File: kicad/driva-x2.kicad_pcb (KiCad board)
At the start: 4 copper layers, 100 x 50 mm, 199 parts, among them J1 CONN_HALL_1, J10 CONN_SPI_2, J11 CONN_CAN, J12 CONN_POWER, J2 CONN_PROG, J3 CONN_USB_OTG, J4 CONN_I2C, J5 CONN_POWER2, J6 CONN_SERVO, J8 CONN_SPI_1, J9 CONN_HALL_2, Q1 TPH1R403NL, Q10 TPH1R403NL, Q11 TPH1R403NL, Q12 TPH1R403NL, Q2 TPH1R403NL, Q3 TPH1R403NL, Q4 TPH1R403NL, Q5 TPH1R403NL, Q6 TPH1R403NL, Q7 TPH1R403NL, Q8 TPH1R403NL, Q9 TPH1R403NL, SW1 push, SW2 push, SW3 push, U1 INA240A2PW, U10 L6387ED, U11 INA240A2PW, U12 L6387ED, U13 AMS1117-3.3, U14 TJA1051T-3, U15 STM32F405RGTx, U2 L6387ED, U3 INA240A2PW, U4 L6387ED, U5 INA240A2PW, U6 L6387ED, U7 INA240A2PW, U8 L6387ED, U9 INA240A2PW

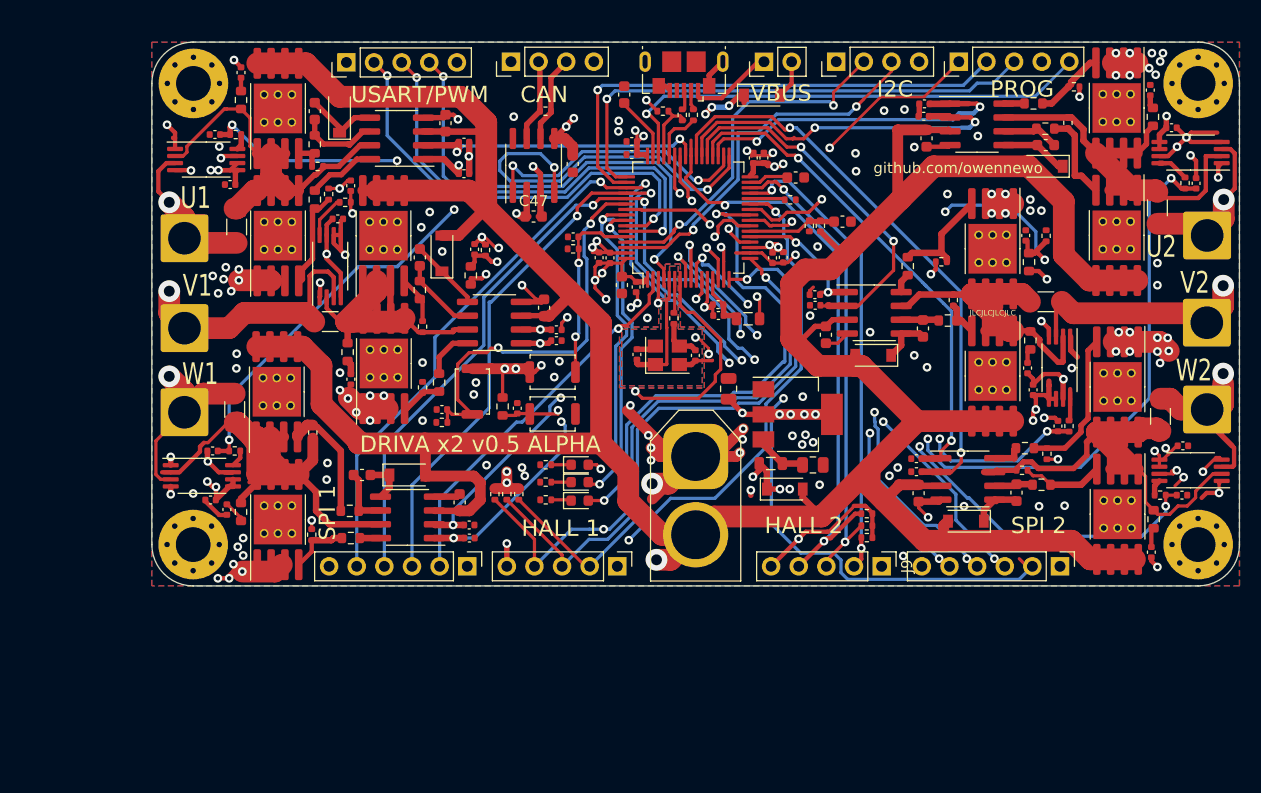
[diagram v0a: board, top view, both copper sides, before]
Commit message: Adding 0.9 version
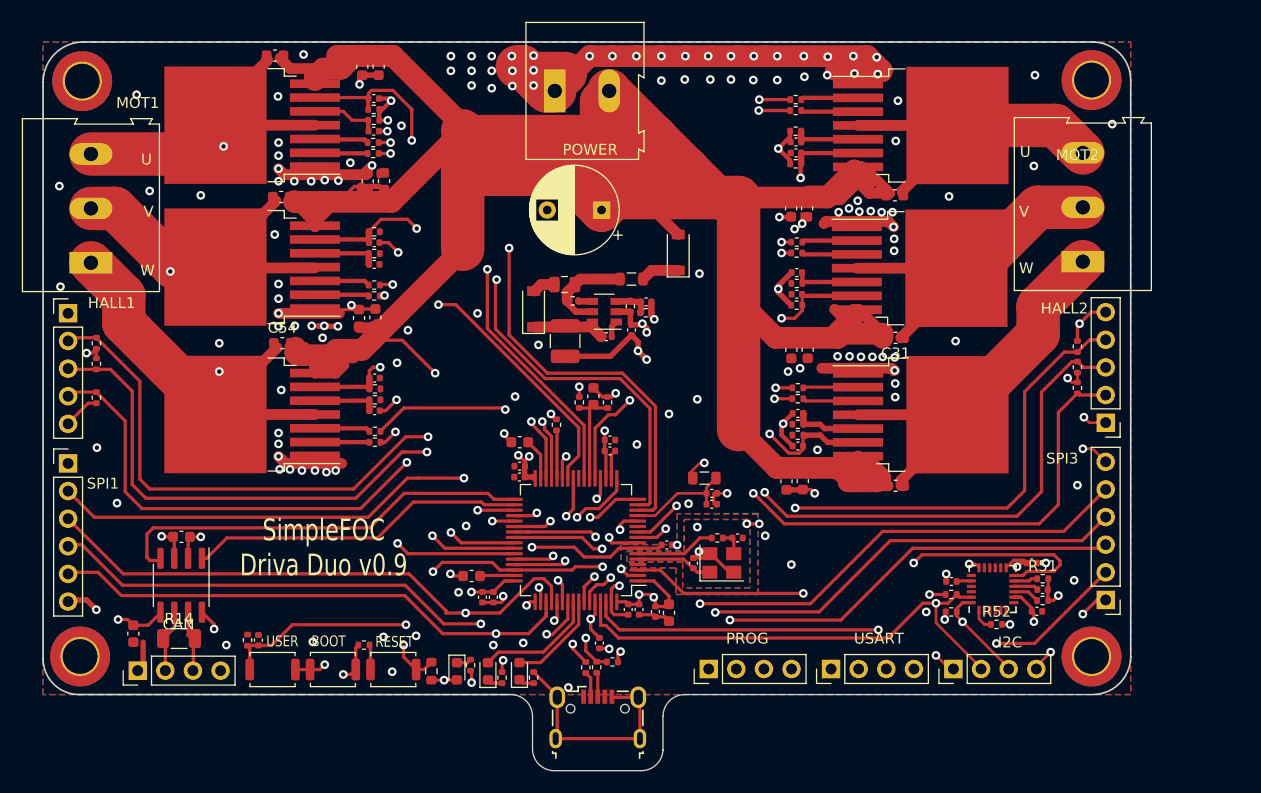
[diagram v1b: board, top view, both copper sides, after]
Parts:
- removed C62, C64, C66, C68: 100n, Capacitor_SMD:C_0402_1005Metric
- removed C63, C65, C67: 1n, Capacitor_SMD:C_0402_1005Metric
- removed D10: BLUE, LED_SMD:LED_0603_1608Metric
- removed D11, D6, D7: b5819w, Diode_SMD:D_SOD-123
- removed D8: RED, LED_SMD:LED_0603_1608Metric
- removed D9: GREEN, LED_SMD:LED_0603_1608Metric
- removed H10: PAD_W_2, Connector_Wire:SolderWire-2.5sqmm_1x01_D2.4mm_OD4.4mm
- removed H5: PAD_U_1, Connector_Wire:SolderWire-2.5sqmm_1x01_D2.4mm_OD4.4mm
- removed H6: PAD_V_1, Connector_Wire:SolderWire-2.5sqmm_1x01_D2.4mm_OD4.4mm
- removed H7: PAD_W_1, Connector_Wire:SolderWire-2.5sqmm_1x01_D2.4mm_OD4.4mm
- removed H8: PAD_U_2, Connector_Wire:SolderWire-2.5sqmm_1x01_D2.4mm_OD4.4mm
- removed H9: PAD_V_2, Connector_Wire:SolderWire-2.5sqmm_1x01_D2.4mm_OD4.4mm
- removed Q1, Q10, Q11, Q12, Q2, Q3, Q4, Q5, Q6, Q7, Q8, Q9: TPH1R403NL, Package_SO:SOP-8-1EP_4.57x4.57mm_P1.27mm_EP4.57x4.45mm_ThermalVias
- removed R53: 3K3, Resistor_SMD:R_0402_1005Metric
- removed R54: 4k7, Resistor_SMD:R_0402_1005Metric
- removed R55: 10k, Resistor_SMD:R_0402_1005Metric
- removed R56, R57, R58, R59, R60, R61, R62, R63, R64: 1K, Resistor_SMD:R_0402_1005Metric
- removed TH1, TH2: Thermistor, Resistor_SMD:R_0603_1608Metric
- removed U11: INA240A2PW, Package_SO:TSSOP-8_4.4x3mm_P0.65mm
- removed U12: L6387ED, Package_SO:SOIC-8_3.9x4.9mm_P1.27mm
- removed U13: AMS1117-3.3, Package_TO_SOT_SMD:SOT-223-3_TabPin2
- removed U14: TJA1051T-3, Package_SO:SOIC-8_3.9x4.9mm_P1.27mm
- removed U15: STM32F405RGTx, Package_QFP:LQFP-64_10x10mm_P0.5mm
- added J7: CONN_SPI_1, Connector_PinHeader_2.54mm:PinHeader_1x06_P2.54mm_Vertical, F.Cu at (64.3, 68.8)
- added L1: 2.2uh, Inductor_SMD:L_1210_3225Metric, F.Cu at (110.0, 57.5)
- C1: value 1u -> 10u
- C10, C20, C25, C30, C5, C53: value 10n -> 100n
- C11, C6: value 1u -> 100n; footprint Capacitor_SMD:C_0603_1608Metric -> Capacitor_SMD:C_0402_1005Metric
- C12: value 100p -> 10u
- C13: value 100p -> 4.7u+; footprint Capacitor_SMD:C_0402_1005Metric -> Capacitor_SMD:C_0805_2012Metric
- C14, C4, C9: value 470n -> 100n; footprint Capacitor_SMD:C_0603_1608Metric -> Capacitor_SMD:C_0402_1005Metric
- C16: value 1u -> 12p; footprint Capacitor_SMD:C_0603_1608Metric -> Capacitor_SMD:C_0402_1005Metric
- C17: value 100p -> 12p
- C18, C2, C3, C7, C8: value 100p -> 100n
- C19: value 470n -> 2.2u
- C21: value 1u -> 2.2u
- C22, C23: value 100p -> 2.2u; footprint Capacitor_SMD:C_0402_1005Metric -> Capacitor_SMD:C_0603_1608Metric
- C24: value 470n -> 10u
- C26: value 1u -> 220n+
- C27: value 100p -> 100n+; footprint Capacitor_SMD:C_0402_1005Metric -> Capacitor_SMD:C_0603_1608Metric
- C28: value 100p -> 220n+; footprint Capacitor_SMD:C_0402_1005Metric -> Capacitor_SMD:C_0603_1608Metric
- C29: value 470n -> 1n; footprint Capacitor_SMD:C_0603_1608Metric -> Capacitor_SMD:C_0402_1005Metric
- C31, C54: value 10u -> 220n+
- C32, C37: value 100n -> 100n+; footprint Capacitor_SMD:C_0402_1005Metric -> Capacitor_SMD:C_0603_1608Metric
- C33, C36, C38, C49, C56: value 100n -> 220n+; footprint Capacitor_SMD:C_0402_1005Metric -> Capacitor_SMD:C_0603_1608Metric
- C34, C39: value 100n -> 1n
- C41, C42: value 10u -> 100n; footprint Capacitor_SMD:C_0805_2012Metric -> Capacitor_SMD:C_0402_1005Metric
- C43: value 100n -> 2.2n
- C44: value 10n -> 220n+; footprint Capacitor_SMD:C_0402_1005Metric -> Capacitor_SMD:C_0603_1608Metric
- C45: value 12p -> 100n+; footprint Capacitor_SMD:C_0402_1005Metric -> Capacitor_SMD:C_0603_1608Metric
- C46: value 12p -> 220n+; footprint Capacitor_SMD:C_0402_1005Metric -> Capacitor_SMD:C_0603_1608Metric
- C47, C52: value 2.2u -> 1n; footprint Capacitor_SMD:C_0603_1608Metric -> Capacitor_SMD:C_0402_1005Metric
- C50: value 2.2u -> 100n+
- C51: value 2.2u -> 220n+
- C55: value 10n -> 100n+; footprint Capacitor_SMD:C_0402_1005Metric -> Capacitor_SMD:C_0603_1608Metric
- C59: value 1n -> 33p
- C60: value 100n -> 1000u+; footprint Capacitor_SMD:C_0402_1005Metric -> Capacitor_THT:CP_Radial_D8.0mm_P5.00mm
- C61: value 1n -> 10n
- D2: value b5819w -> RED; footprint Diode_SMD:D_SOD-123 -> LED_SMD:LED_0603_1608Metric
- D3: value b5819w -> GREEN; footprint Diode_SMD:D_SOD-123 -> LED_SMD:LED_0603_1608Metric
- D4: value b5819w -> BLUE; footprint Diode_SMD:D_SOD-123 -> LED_SMD:LED_0603_1608Metric
- H1, H2, H3, H4: footprint MountingHole:MountingHole_3.2mm_M3_Pad_Via -> MountingHole:MountingHole_3.2mm_M3_ISO14580_Pad_TopBottom
- J10: value CONN_SPI_2 -> CONN_CAN; footprint Connector_PinHeader_2.54mm:PinHeader_1x06_P2.54mm_Vertical -> Connector_PinHeader_2.54mm:PinHeader_1x04_P2.54mm_Vertical
- J11: value CONN_CAN -> CONN_PWR; footprint Connector_PinHeader_2.54mm:PinHeader_1x04_P2.54mm_Vertical -> TerminalBlock:TerminalBlock_Altech_AK300-2_P5.00mm
- J12: value CONN_POWER -> CONN_SERIAL; footprint Connector_AMASS:AMASS_XT60-M_1x02_P7.20mm_Vertical -> Connector_PinHeader_2.54mm:PinHeader_1x04_P2.54mm_Vertical
- J2: footprint Connector_PinHeader_2.54mm:PinHeader_1x05_P2.54mm_Vertical -> Connector_PinHeader_2.54mm:PinHeader_1x04_P2.54mm_Vertical
- J3: footprint Connector_USB:USB_Micro-B_GCT_USB3076-30-A -> Connector_USB:USB_Micro-B_Wuerth_629105150521
- J4: value CONN_I2C -> CONN_MOT_1; footprint Connector_PinHeader_2.54mm:PinHeader_1x04_P2.54mm_Vertical -> TerminalBlock:TerminalBlock_Altech_AK300-3_P5.00mm
- J5: value CONN_POWER2 -> CONN_SERIAL; footprint Connector_PinHeader_2.54mm:PinHeader_1x02_P2.54mm_Vertical -> Connector_PinHeader_2.54mm:PinHeader_1x04_P2.54mm_Vertical
- J6: value CONN_SERVO -> CONN_MOT_2; footprint Connector_PinHeader_2.54mm:PinHeader_1x05_P2.54mm_Vertical -> TerminalBlock:TerminalBlock_Altech_AK300-3_P5.00mm
- J8: value CONN_SPI_1 -> CONN_SPI_2
- R10: value 33 -> 220; footprint Resistor_SMD:R_0603_1608Metric -> Resistor_SMD:R_0402_1005Metric
- R11: value 10k -> 2K2; footprint Resistor_SMD:R_0402_1005Metric -> Resistor_SMD:R_0603_1608Metric
- R12, R30, R42: value 0.002R @1W -> 10k; footprint Resistor_SMD:R_1206_3216Metric -> Resistor_SMD:R_0402_1005Metric
- R13, R22, R25, R34, R37: value 33 -> 10k; footprint Resistor_SMD:R_0603_1608Metric -> Resistor_SMD:R_0402_1005Metric
- R14: value 1 -> 120R+; footprint Resistor_SMD:R_0603_1608Metric -> Resistor_SMD:R_1206_3216Metric
- R15: value 10k -> 33K
- R16: value 33 -> 3K3; footprint Resistor_SMD:R_0603_1608Metric -> Resistor_SMD:R_0402_1005Metric
- R18: value 0.002R @1W -> 1K; footprint Resistor_SMD:R_1206_3216Metric -> Resistor_SMD:R_0402_1005Metric
- R19: value 33 -> 1K; footprint Resistor_SMD:R_0603_1608Metric -> Resistor_SMD:R_0402_1005Metric
- R20: value 1 -> 1K; footprint Resistor_SMD:R_0603_1608Metric -> Resistor_SMD:R_0402_1005Metric
- R23, R27, R35, R39: value 10k -> 1k
- R24, R36: value 0.002R @1W -> 510R; footprint Resistor_SMD:R_1206_3216Metric -> Resistor_SMD:R_0402_1005Metric
- R26, R38: value 1 -> 10k; footprint Resistor_SMD:R_0603_1608Metric -> Resistor_SMD:R_0402_1005Metric
- R28, R40: value 33 -> 510R; footprint Resistor_SMD:R_0603_1608Metric -> Resistor_SMD:R_0402_1005Metric
- R31, R43: value 33 -> 1k; footprint Resistor_SMD:R_0603_1608Metric -> Resistor_SMD:R_0402_1005Metric
- R32, R44: value 1 -> 510R; footprint Resistor_SMD:R_0603_1608Metric -> Resistor_SMD:R_0402_1005Metric
- R45: value 10k -> 400K
- R46: value 220 -> 4.7k
- R47: value 2K2 -> 4.7k; footprint Resistor_SMD:R_0603_1608Metric -> Resistor_SMD:R_0402_1005Metric
- R48: value 10k -> 4.7k
- R49: value 10k -> 120k
- R50: value 220 -> 39k
- R51: value 33K -> 10k
- R52: value 4k7 -> 10k
- U1: value INA240A2PW -> mp2451dt; footprint Package_SO:TSSOP-8_4.4x3mm_P0.65mm -> Package_TO_SOT_SMD:SOT-23-6
- U10, U4, U6, U8: value L6387ED -> IFX007T; footprint Package_SO:SOIC-8_3.9x4.9mm_P1.27mm -> Package_TO_SOT_SMD:TO-263-7_TabPin8
- U2: value L6387ED -> TJA1051T-3
- U3: value INA240A2PW -> STM32F405RGTx; footprint Package_SO:TSSOP-8_4.4x3mm_P0.65mm -> Package_QFP:LQFP-64_10x10mm_P0.5mm
- U5, U9: value INA240A2PW -> IFX007T; footprint Package_SO:TSSOP-8_4.4x3mm_P0.65mm -> Package_TO_SOT_SMD:TO-263-7_TabPin8
- U7: value INA240A2PW -> MPU-6050; footprint Package_SO:TSSOP-8_4.4x3mm_P0.65mm -> Sensor_Motion:InvenSense_QFN-24_4x4mm_P0.5mm
- moved H1 102.6 mm to (65.6, 33.6)
- moved R14 101.6 mm to (74.5, 84.8), turned to 0 degrees
- moved H3 98.0 mm to (158.4, 86.5)
- moved J10 85.3 mm to (70.7, 87.8), turned to 90 degrees
- moved U2 84.6 mm to (74.7, 80.0), turned to 270 degrees
- moved U7 82.4 mm to (149.3, 80.3), turned to 90 degrees
- moved R13 79.2 mm to (91.5, 85.5)
- moved C58 77.8 mm to (92.5, 63.9)
- moved C57 77.6 mm to (92.5, 60.9), turned to 0 degrees
- moved R11 77.2 mm to (97.7, 87.8)
- moved C5 77.1 mm to (102.4, 81.0)
- moved R17 72.0 mm to (80.8, 85.0), turned to 90 degrees
- moved J4 71.0 mm to (66.4, 50.3)
- moved J6 70.1 mm to (157.6, 50.2)
- moved R18 62.6 mm to (101.3, 87.3), turned to 90 degrees
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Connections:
- C1 pad 1: Net-(C1-Pad1) -> GND
- C1 pad 2: Net-(C1-Pad2) -> +3V3
- C10 pad 1: Net-(C10-Pad1) -> GND
- C10 pad 2: GND -> +3V3
- C12 pad 1: /driver_2/HIN_W -> GND
- C12 pad 2: GND -> +3V3
- C13 pad 1: /driver_2/LIN_W -> GND
- C13 pad 2: GND -> Net-(C13-Pad2)
- C14 pad 1: VCC -> GND
- C14 pad 2: GND -> +3.3VA
- C15 pad 1: Net-(C15-Pad1) -> GND
- C15 pad 2: GND -> +3.3VA
- C16 pad 1: Net-(C16-Pad1) -> HSE_IN
- C16 pad 2: Net-(C16-Pad2) -> GND
- C17 pad 1: /driver_1/HIN_U -> Net-(C17-Pad1)
- C18 pad 1: /driver_1/LIN_U -> BOOT0
- C19 pad 1: VCC -> GND
- C19 pad 2: GND -> +3V3
- C2 pad 1: /driver_2/HIN_U -> GND
- C2 pad 2: GND -> +3V3
- C20 pad 1: Net-(C20-Pad1) -> NRST
- C21 pad 1: Net-(C21-Pad1) -> GND
- C21 pad 2: Net-(C21-Pad2) -> +3V3
- C22 pad 1: /driver_1/HIN_V -> Net-(C22-Pad1)
- C23 pad 1: /driver_1/LIN_V -> Net-(C23-Pad1)
- C24 pad 1: VCC -> GND
- C24 pad 2: GND -> BATTERY
- C25 pad 1: Net-(C25-Pad1) -> USER_BUTTON
- C26 pad 1: Net-(C26-Pad1) -> /driver-2/OUT_U
- C26 pad 2: Net-(C26-Pad2) -> VCC
- C27 pad 1: /driver_1/HIN_W -> VCC
- C28 pad 1: /driver_1/LIN_W -> VCC
- C29 pad 1: VCC -> /driver-2/SENSE_U
- C3 pad 1: /driver_2/LIN_U -> GND
- C3 pad 2: GND -> +3V3
- C31 pad 1: GND -> /driver-2/OUT_V
- C31 pad 2: +3V3 -> VCC
- C32 pad 1: GND -> VCC
- C32 pad 2: +3V3 -> GND
- C33 pad 1: GND -> VCC
- C33 pad 2: +3V3 -> GND
- C34 pad 1: GND -> /driver-2/SENSE_V
- C34 pad 2: +3V3 -> GND
- C35 pad 1: GND -> Net-(C35-Pad1)
- C35 pad 2: +3V3 -> GND
- C36 pad 1: GND -> /driver-2/OUT_W
- C36 pad 2: +3V3 -> VCC
- C37 pad 1: GND -> VCC
- C37 pad 2: +3V3 -> GND
- C38 pad 1: GND -> VCC
- C38 pad 2: +3V3 -> GND
- C39 pad 1: GND -> /driver-2/SENSE_W
- C39 pad 2: +3V3 -> GND
- C4 pad 1: VCC -> GND
- C4 pad 2: GND -> +3V3
- C40 pad 1: GND -> Net-(C40-Pad1)
- C40 pad 2: +3V3 -> GND
- C41 pad 2: Net-(C41-Pad2) -> +3V3
- C42 pad 2: +3V3 -> Net-(C42-Pad2)
- C43 pad 2: +3.3VA -> Net-(C43-Pad2)
- C44 pad 1: GND -> /driver-1/OUT_U
- C44 pad 2: +3.3VA -> VCC
- C45 pad 1: HSE_IN -> VCC
- C46 pad 1: Net-(C46-Pad1) -> VCC
- C47 pad 1: GND -> /driver-1/SENSE_U
- C47 pad 2: +3V3 -> GND
- C48 pad 1: BOOT0 -> Net-(C48-Pad1)
- C49 pad 1: NRST -> /driver-1/OUT_V
- C49 pad 2: GND -> VCC
- C5 pad 1: Net-(C5-Pad1) -> GND
- C5 pad 2: GND -> +3V3
- C50 pad 1: GND -> VCC
- C50 pad 2: +3V3 -> GND
- C51 pad 1: Net-(C51-Pad1) -> VCC
- C52 pad 1: Net-(C52-Pad1) -> /driver-1/SENSE_V
- C53 pad 1: TEMP_1 -> Net-(C53-Pad1)
- C54 pad 1: GND -> /driver-1/OUT_W
- C54 pad 2: BATTERY -> VCC
- C55 pad 1: TEMP_2 -> VCC
- C56 pad 1: USER_BUTTON -> VCC
- C57 pad 1: /driver_2/SENSE_U -> /driver-1/SENSE_W
- C58 pad 1: +3V3 -> Net-(C58-Pad1)
- C59 pad 1: /driver_2/SENSE_V -> Net-(C59-Pad1)
- C59 pad 2: GND -> +3V3
- C6 pad 1: Net-(C6-Pad1) -> GND
- C6 pad 2: Net-(C6-Pad2) -> +3V3
- C60 pad 1: +3V3 -> VCC
- C61 pad 1: /driver_2/SENSE_W -> +3V3
- C7 pad 1: /mcu/HIN_U_2 -> GND
- C7 pad 2: GND -> +3V3
- C8 pad 1: /mcu/LIN_U_2 -> GND
- C8 pad 2: GND -> +3V3
- C9 pad 1: VCC -> GND
- C9 pad 2: GND -> +3V3
- D1 pad 1: Net-(C1-Pad2) -> Net-(D1-Pad1)
- D2 pad 1: Net-(C6-Pad2) -> Net-(D2-Pad1)
- D2 pad 2: VCC -> +3V3
- D3 pad 1: Net-(C11-Pad2) -> Net-(D3-Pad1)
- D3 pad 2: VCC -> LED_GREEN
- D4 pad 1: Net-(C16-Pad2) -> Net-(D4-Pad1)
- D4 pad 2: VCC -> LED_BLUE
- D5 pad 1: Net-(C21-Pad2) -> Net-(C11-Pad1)
- D5 pad 2: VCC -> GND
- FB1 pad 1: Net-(C41-Pad2) -> Net-(C13-Pad2)
- FB1 pad 2: Net-(D11-Pad1) -> Net-(D1-Pad1)
- HSE1 pad 3: Net-(C46-Pad1) -> Net-(C17-Pad1)
- J1 pad 2: /mcu/HALL_U_1 -> /mcu/HALL_U1
- J1 pad 3: /mcu/HALL_V_1 -> /mcu/HALL_V1
- J1 pad 4: /mcu/HALL_W_1 -> /mcu/HALL_W1
- J10 pad 2: /mcu/SPI3_SS2 -> /mcu/CAN_L
- J10 pad 3: /mcu/SPI3_MISO -> /mcu/CAN_H
- J10 pad 4: /mcu/SPI3_MOSI -> +3V3
- J11 pad 2: /mcu/CAN_H -> VCC
- J12 pad 2: VCC -> /mcu/I2C1_SCL
- J2 pad 1: /mcu/JTAG_DO -> /mcu/SWO
- J2 pad 2: /mcu/JTAG_DI -> /mcu/SWCLK
- J2 pad 3: /mcu/SWCLK -> GND
- J2 pad 4: GND -> /mcu/SWDIO
- J4 pad 1: GND -> /driver-1/OUT_W
- J4 pad 2: /mcu/I2C_1_SCL -> /driver-1/OUT_V
- J4 pad 3: /mcu/I2C_1_SDA -> /driver-1/OUT_U
- J5 pad 1: Net-(J3-Pad1) -> GND
- J5 pad 2: ALT_POWER -> /mcu/USART1_TX
- J6 pad 1: GND -> /driver-2/OUT_W
- J6 pad 2: /mcu/USART1_TX -> /driver-2/OUT_V
- J6 pad 3: /mcu/USART1_RX -> /driver-2/OUT_U
- J8 pad 2: /mcu/SPI3_SS1 -> /mcu/SPI3_SS2
- J8 pad 3: /mcu/SPI3_MISO -> SPI3_MOSI
- J8 pad 4: /mcu/SPI3_MOSI -> SPI3_MISO
- J8 pad 5: /mcu/SPI3_SCLK -> SPI3_SCLK
- J9 pad 2: /mcu/HALL_U_I2C_2_SCL -> /mcu/HALL_U2
- J9 pad 3: /mcu/HALL_V_I2C_2_SDA -> /mcu/HALL_V2
- J9 pad 4: /mcu/HALL_W_2 -> /mcu/HALL_W2
- R10 pad 1: Net-(Q1-Pad4) -> HSE_OUT
- R10 pad 2: Net-(C1-Pad1) -> Net-(C17-Pad1)
- R11 pad 1: Net-(Q1-Pad1) -> NRST
- R11 pad 2: Net-(Q1-Pad4) -> +3V3
- R12 pad 1: /driver_2/OUT_U -> GND
- R12 pad 2: Net-(Q1-Pad1) -> BOOT1
- R13 pad 1: Net-(Q2-Pad4) -> GND
- R13 pad 2: Net-(R13-Pad2) -> BOOT0
- R14 pad 1: Net-(C5-Pad1) -> /mcu/CAN_L
- R14 pad 2: Net-(Q1-Pad1) -> /mcu/CAN_H
- R15 pad 1: GND -> BATTERY
- R15 pad 2: Net-(Q2-Pad4) -> VCC
- R16 pad 1: Net-(Q3-Pad4) -> GND
- R16 pad 2: Net-(C6-Pad1) -> BATTERY
- R17 pad 1: Net-(Q3-Pad1) -> USER_BUTTON
- R17 pad 2: Net-(Q3-Pad4) -> GND
- R18 pad 1: /driver_2/OUT_V -> GND
- R18 pad 2: Net-(Q3-Pad1) -> Net-(D2-Pad1)
- R19 pad 1: Net-(Q4-Pad4) -> GND
- R19 pad 2: Net-(R19-Pad2) -> Net-(D3-Pad1)
- R20 pad 1: Net-(C10-Pad1) -> GND
- R20 pad 2: Net-(Q3-Pad1) -> Net-(D4-Pad1)
- R21 pad 1: GND -> Net-(R21-Pad1)
- R21 pad 2: Net-(Q4-Pad4) -> /driver-2/IN_U
- R22 pad 1: Net-(Q5-Pad4) -> Net-(R22-Pad1)
- R22 pad 2: Net-(C11-Pad1) -> /driver-2/EN_U
- R23 pad 1: Net-(Q5-Pad1) -> /driver-2/SENSE_U
- R23 pad 2: Net-(Q5-Pad4) -> GND
- R24 pad 1: /driver_2/OUT_W -> Net-(C30-Pad1)
- R24 pad 2: Net-(Q5-Pad1) -> GND
- R25 pad 1: Net-(Q6-Pad4) -> Net-(R25-Pad1)
- R25 pad 2: Net-(R25-Pad2) -> /driver-2/IN_V
- R26 pad 1: Net-(C15-Pad1) -> Net-(R26-Pad1)
- R26 pad 2: Net-(Q5-Pad1) -> /driver-2/EN_V
- R27 pad 1: GND -> /driver-2/SENSE_V
- R27 pad 2: Net-(Q6-Pad4) -> GND
- R28 pad 1: Net-(Q7-Pad4) -> Net-(C35-Pad1)
- R28 pad 2: Net-(C16-Pad1) -> GND
- R29 pad 1: Net-(Q7-Pad1) -> Net-(R29-Pad1)
- R29 pad 2: Net-(Q7-Pad4) -> /driver-2/IN_W
- R30 pad 1: /driver_1/OUT_U -> Net-(R30-Pad1)
- R30 pad 2: Net-(Q7-Pad1) -> /driver-2/EN_W
- R31 pad 1: Net-(Q8-Pad4) -> /driver-2/SENSE_W
- R31 pad 2: Net-(R31-Pad2) -> GND
- R32 pad 1: Net-(C20-Pad1) -> Net-(C40-Pad1)
- R32 pad 2: Net-(Q7-Pad1) -> GND
- R33 pad 1: GND -> Net-(R33-Pad1)
- R33 pad 2: Net-(Q8-Pad4) -> /driver-1/IN_U
- R34 pad 1: Net-(Q9-Pad4) -> Net-(R34-Pad1)
- R34 pad 2: Net-(C21-Pad1) -> /driver-1/EN_U
- R35 pad 1: Net-(Q10-Pad5) -> /driver-1/SENSE_U
- R35 pad 2: Net-(Q9-Pad4) -> GND
- R36 pad 1: /driver_1/OUT_V -> Net-(C48-Pad1)
- R36 pad 2: Net-(Q10-Pad5) -> GND
- R37 pad 1: Net-(Q10-Pad4) -> Net-(R37-Pad1)
- R37 pad 2: Net-(R37-Pad2) -> /driver-1/IN_V
- R38 pad 1: Net-(C25-Pad1) -> Net-(R38-Pad1)
- R38 pad 2: Net-(Q10-Pad5) -> /driver-1/EN_V
- R39 pad 1: GND -> /driver-1/SENSE_V
- R39 pad 2: Net-(Q10-Pad4) -> GND
- R4 pad 2: /mcu/HALL_W_1 -> /mcu/HALL_W1
- R40 pad 1: Net-(Q11-Pad4) -> Net-(C53-Pad1)
- R40 pad 2: Net-(C26-Pad1) -> GND
- R41 pad 1: Net-(Q11-Pad1) -> Net-(R41-Pad1)
- R41 pad 2: Net-(Q11-Pad4) -> /driver-1/IN_W
- R42 pad 1: /driver_1/OUT_W -> Net-(R42-Pad1)
- R42 pad 2: Net-(Q11-Pad1) -> /driver-1/EN_W
- R43 pad 1: Net-(Q12-Pad4) -> /driver-1/SENSE_W
- R43 pad 2: Net-(R43-Pad2) -> GND
- R44 pad 1: Net-(C30-Pad1) -> Net-(C58-Pad1)
- R44 pad 2: Net-(Q11-Pad1) -> GND
- R45 pad 1: GND -> Net-(R45-Pad1)
- R45 pad 2: Net-(Q12-Pad4) -> Net-(C13-Pad2)
- R46 pad 1: HSE_OUT -> +3V3
- R46 pad 2: Net-(C46-Pad1) -> /mcu/I2C1_SCL
- R47 pad 1: NRST -> +3V3
- R47 pad 2: +3V3 -> /mcu/I2C1_SDA
- R48 pad 1: GND -> Net-(R48-Pad1)
- R48 pad 2: BOOT1 -> GND
- R49 pad 1: GND -> +3V3
- R49 pad 2: BOOT0 -> Net-(C59-Pad1)
- R5 pad 2: /mcu/HALL_V_1 -> /mcu/HALL_V1
- R50 pad 1: /mcu/CAN_L -> Net-(C59-Pad1)
- R50 pad 2: /mcu/CAN_H -> GND
- R51 pad 1: BATTERY -> Net-(R51-Pad1)
- R51 pad 2: VCC -> GND
- R52 pad 1: GND -> Net-(R52-Pad1)
- R52 pad 2: TEMP_1 -> GND
- R6 pad 2: /mcu/HALL_U_1 -> /mcu/HALL_U1
- R7 pad 2: /mcu/HALL_W_2 -> /mcu/HALL_W2
- R8 pad 2: /mcu/HALL_V_I2C_2_SDA -> /mcu/HALL_V2
- R9 pad 2: /mcu/HALL_U_I2C_2_SCL -> /mcu/HALL_U2
- U1 pad 1: GND -> Net-(C11-Pad2)
- U1 pad 2: Net-(Q1-Pad1) -> GND
- U1 pad 3: /driver_2/OUT_U -> Net-(C59-Pad1)
- U1 pad 4: GND -> Net-(R45-Pad1)
- U1 pad 5: +3V3 -> Net-(C13-Pad2)
- U1 pad 6: +3V3 -> Net-(C11-Pad1)
- U10 pad 1: /driver_1/LIN_V -> GND
- U10 pad 2: /driver_1/HIN_V -> Net-(R41-Pad1)
- U10 pad 3: VCC -> Net-(R42-Pad1)
- U10 pad 4: GND -> /driver-1/OUT_W
- U10 pad 5: Net-(C21-Pad2) -> Net-(C58-Pad1)
- U10 pad 6: Net-(C21-Pad1) -> /driver-1/SENSE_W
- U10 pad 7: Net-(Q10-Pad5) -> VCC
- U10 pad 8: Net-(R37-Pad2) -> /driver-1/OUT_W
- U2 pad 1: /driver_2/LIN_U -> CAN2_TX
- U2 pad 2: /driver_2/HIN_U -> GND
- U2 pad 3: VCC -> +3V3
- U2 pad 4: GND -> CAN2_RX
- U2 pad 5: Net-(C1-Pad2) -> +3V3
- U2 pad 6: Net-(C1-Pad1) -> /mcu/CAN_L
- U2 pad 7: Net-(Q1-Pad1) -> /mcu/CAN_H
- U2 pad 8: Net-(R13-Pad2) -> GND
- U3 pad 1: GND -> +3V3
- U3 pad 2: Net-(Q3-Pad1) -> /mcu/SPI3_SS1
- U3 pad 3: /driver_2/OUT_V -> /mcu/SPI3_SS2
- U3 pad 4: GND -> Net-(U3-Pad4)
- U3 pad 5: +3V3 -> HSE_IN
- U3 pad 6: +3V3 -> HSE_OUT
- U3 pad 7: GND -> NRST
- U3 pad 8: Net-(R60-Pad2) -> /driver-2/SENSE_U
- U4 pad 1: /mcu/LIN_U_2 -> GND
- U4 pad 2: /mcu/HIN_U_2 -> Net-(R21-Pad1)
- U4 pad 3: VCC -> Net-(R22-Pad1)
- U4 pad 4: GND -> /driver-2/OUT_U
- U4 pad 5: Net-(C6-Pad2) -> Net-(C30-Pad1)
- U4 pad 6: Net-(C6-Pad1) -> /driver-2/SENSE_U
- U4 pad 7: Net-(Q3-Pad1) -> VCC
- U4 pad 8: Net-(R19-Pad2) -> /driver-2/OUT_U
- U5 pad 2: Net-(Q5-Pad1) -> Net-(R25-Pad1)
- U5 pad 3: /driver_2/OUT_W -> Net-(R26-Pad1)
- U5 pad 4: GND -> /driver-2/OUT_V
- U5 pad 5: +3V3 -> Net-(C35-Pad1)
- U5 pad 6: +3V3 -> /driver-2/SENSE_V
- U5 pad 7: GND -> VCC
- U5 pad 8: Net-(R61-Pad2) -> /driver-2/OUT_V
- U6 pad 1: /driver_2/LIN_W -> GND
- U6 pad 2: /driver_2/HIN_W -> Net-(R29-Pad1)
- U6 pad 3: VCC -> Net-(R30-Pad1)
- U6 pad 4: GND -> /driver-2/OUT_W
- U6 pad 5: Net-(C11-Pad2) -> Net-(C40-Pad1)
- U6 pad 6: Net-(C11-Pad1) -> /driver-2/SENSE_W
- U6 pad 7: Net-(Q5-Pad1) -> VCC
- U6 pad 8: Net-(R25-Pad2) -> /driver-2/OUT_W
- U7 pad 1: GND -> Net-(R52-Pad1)
- U7 pad 2: Net-(Q7-Pad1) -> (no net)
- U7 pad 3: /driver_1/OUT_U -> (no net)
- U7 pad 4: GND -> (no net)
- U7 pad 5: +3V3 -> (no net)
- U7 pad 6: +3V3 -> Net-(U7-Pad6)
- U7 pad 7: GND -> Net-(U7-Pad7)
- U7 pad 8: Net-(R62-Pad2) -> +3V3
- U8 pad 1: /driver_1/LIN_U -> GND
- U8 pad 2: /driver_1/HIN_U -> Net-(R33-Pad1)
- U8 pad 3: VCC -> Net-(R34-Pad1)
- U8 pad 4: GND -> /driver-1/OUT_U
- U8 pad 5: Net-(C16-Pad2) -> Net-(C48-Pad1)
- U8 pad 6: Net-(C16-Pad1) -> /driver-1/SENSE_U
- U8 pad 7: Net-(Q7-Pad1) -> VCC
- U8 pad 8: Net-(R31-Pad2) -> /driver-1/OUT_U
- U9 pad 2: Net-(Q10-Pad5) -> Net-(R37-Pad1)
- U9 pad 3: /driver_1/OUT_V -> Net-(R38-Pad1)
- U9 pad 4: GND -> /driver-1/OUT_V
- U9 pad 5: +3V3 -> Net-(C53-Pad1)
- U9 pad 6: +3V3 -> /driver-1/SENSE_V
- U9 pad 7: GND -> VCC
- U9 pad 8: Net-(R63-Pad2) -> /driver-1/OUT_V
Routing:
- net SPI3_MOSI: track 0.00 -> 120.6 mm, vias 0 -> 2
- net SPI3_MISO: track 0.00 -> 116.2 mm, vias 0 -> 3
- net SPI3_SCLK: track 0.00 -> 111.8 mm, vias 0 -> 2
- net Net-(D11-Pad1): track 110.4 -> 0.00 mm, vias 7 -> 0
- net /mcu/SPI3_SCLK: track 103.4 -> 0.00 mm, vias 5 -> 0
- net /mcu/SPI3_MOSI: track 101.4 -> 0.00 mm, vias 5 -> 0
- net /mcu/SPI3_MISO: track 101.3 -> 0.00 mm, vias 5 -> 0
- net /driver_2/SENSE_U: track 81.6 -> 0.00 mm, vias 4 -> 0
- net /mcu/HALL_V2: track 0.00 -> 75.4 mm, vias 0 -> 2
- net /driver_1/LIN_W: track 75.2 -> 0.00 mm, vias 4 -> 0
- net /mcu/HALL_U2: track 0.00 -> 71.7 mm, vias 0 -> 2
- net /mcu/HALL_U1: track 0.00 -> 69.6 mm, vias 0 -> 2
- net /mcu/HALL_W2: track 0.00 -> 69.0 mm, vias 0 -> 2
- net /driver_1/SENSE_W: track 67.7 -> 0.00 mm, vias 3 -> 0
- net /mcu/HALL_V1: track 0.00 -> 67.2 mm, vias 0 -> 2
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- added copper zone on B.Cu, net +3V3
- added copper zone on In2.Cu, net GND
- removed copper zone on In2.Cu, net +3V3
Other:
- board size 100 x 50 mm -> 100 x 67 mm
- board text added: "+"
- board text added: "-"
- board text added: "BOOT"
- board text added: "HALL1"
- board text added: "HALL2"
- board text added: "HALL_U1"
- board text added: "HALL_U2"
- board text added: "HALL_V1"
- board text added: "HALL_V2"
- board text added: "HALL_W1"
- board text added: "HALL_W2"
- board text added: "MOT1"
- board text added: "MOT2"
- board text added: "POWER"
- board text added: "RESET"
- board text added: "SPI1"
- board text added: "SPI3"
- board text added: "SWO"
- board text added: "SimpleFOC Driva Duo v0.9"
- board text added: "U"
- board text added: "USART"
- board text added: "USER"
- board text added: "V"
- board text added: "VCC"
- board text added: "W"
- board text removed: "DANGER !"
- board text removed: "DRIVA x2 v0.5 ALPHA"
- board text removed: "HALL 1"
- board text removed: "HALL 2"
- board text removed: "HALL_U_1"
- board text removed: "HALL_V_1"
- board text removed: "HALL_W_1"
- board text removed: "HALL_W_2"
- board text removed: "JLCJLCJLCJLC"
- board text removed: "JTAG_DI"
- board text removed: "JTAG_DO"
- board text removed: "SCL_HALL_U_2"
- board text removed: "SDA_HALL_V_2"
- board text removed: "SERVO"
- board text removed: "SPI 1"
- board text removed: "SPI 2"
- board text removed: "U1"
- board text removed: "U2"
- board text removed: "USART/PWM"
- board text removed: "USB OTG"
- board text removed: "V1"
- board text removed: "V2"
- board text removed: "VBUS"
- board text removed: "VBUS 5V"
- board text removed: "W1"
- board text removed: "W2"
- board text removed: "github.com/owennewo"
